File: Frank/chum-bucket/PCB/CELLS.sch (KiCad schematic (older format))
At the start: 8 parts, among them U207 CM, U208 CM, U209 CM, U210 CM, U211 CM, U212 CM, U213 CM, U214 CM

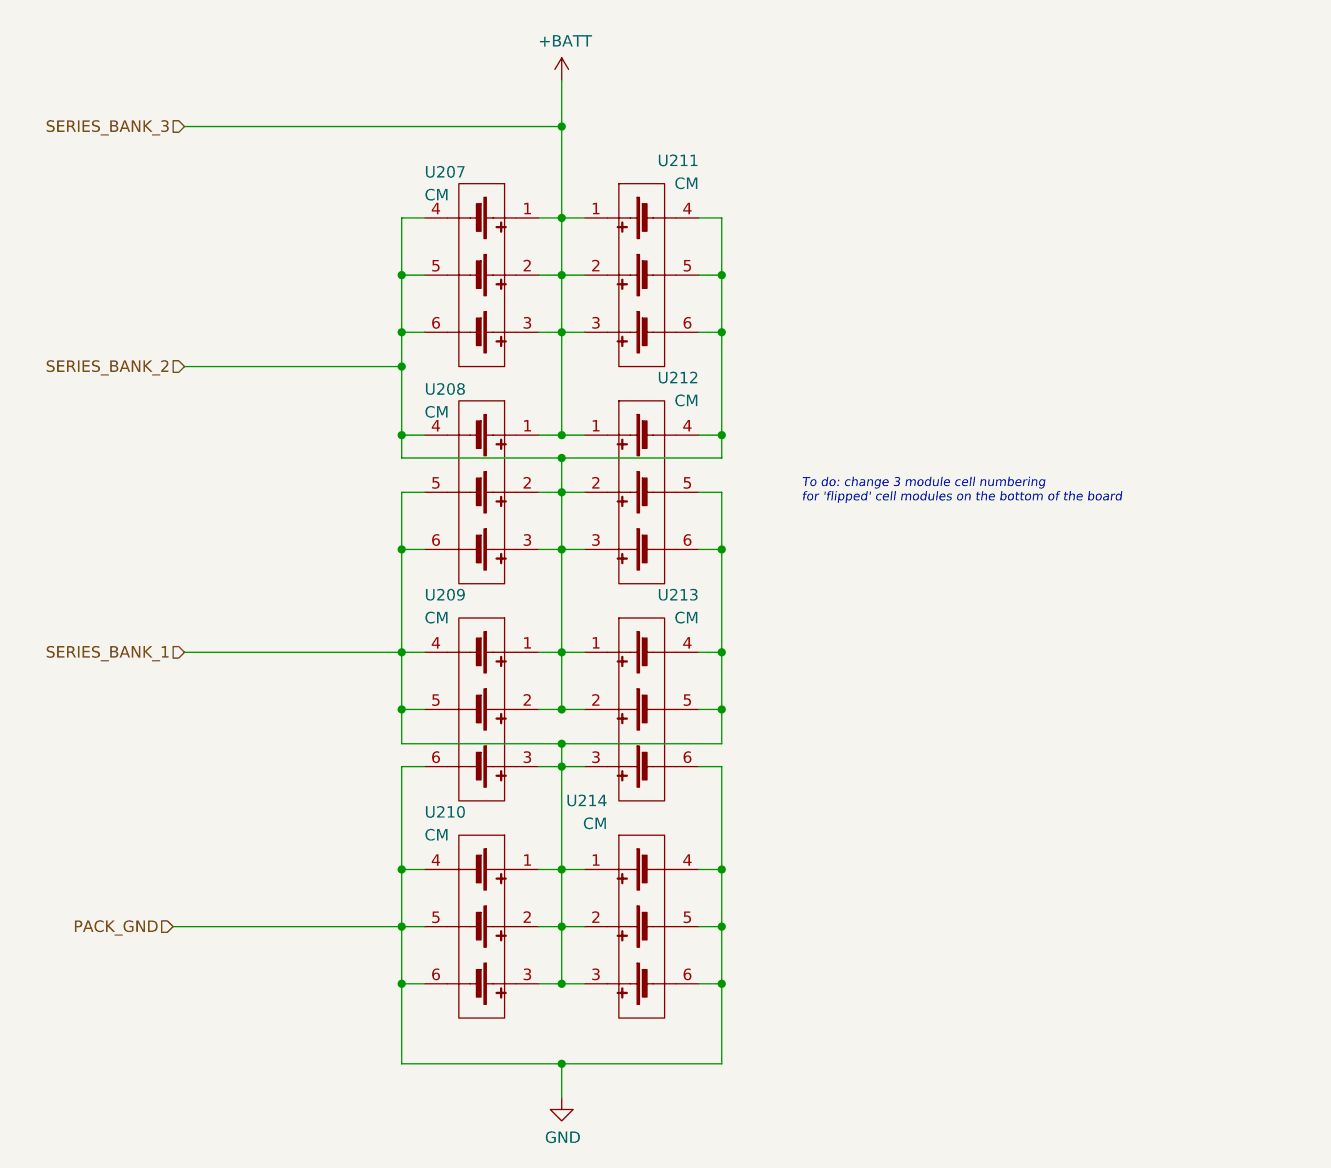
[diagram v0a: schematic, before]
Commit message: some layout
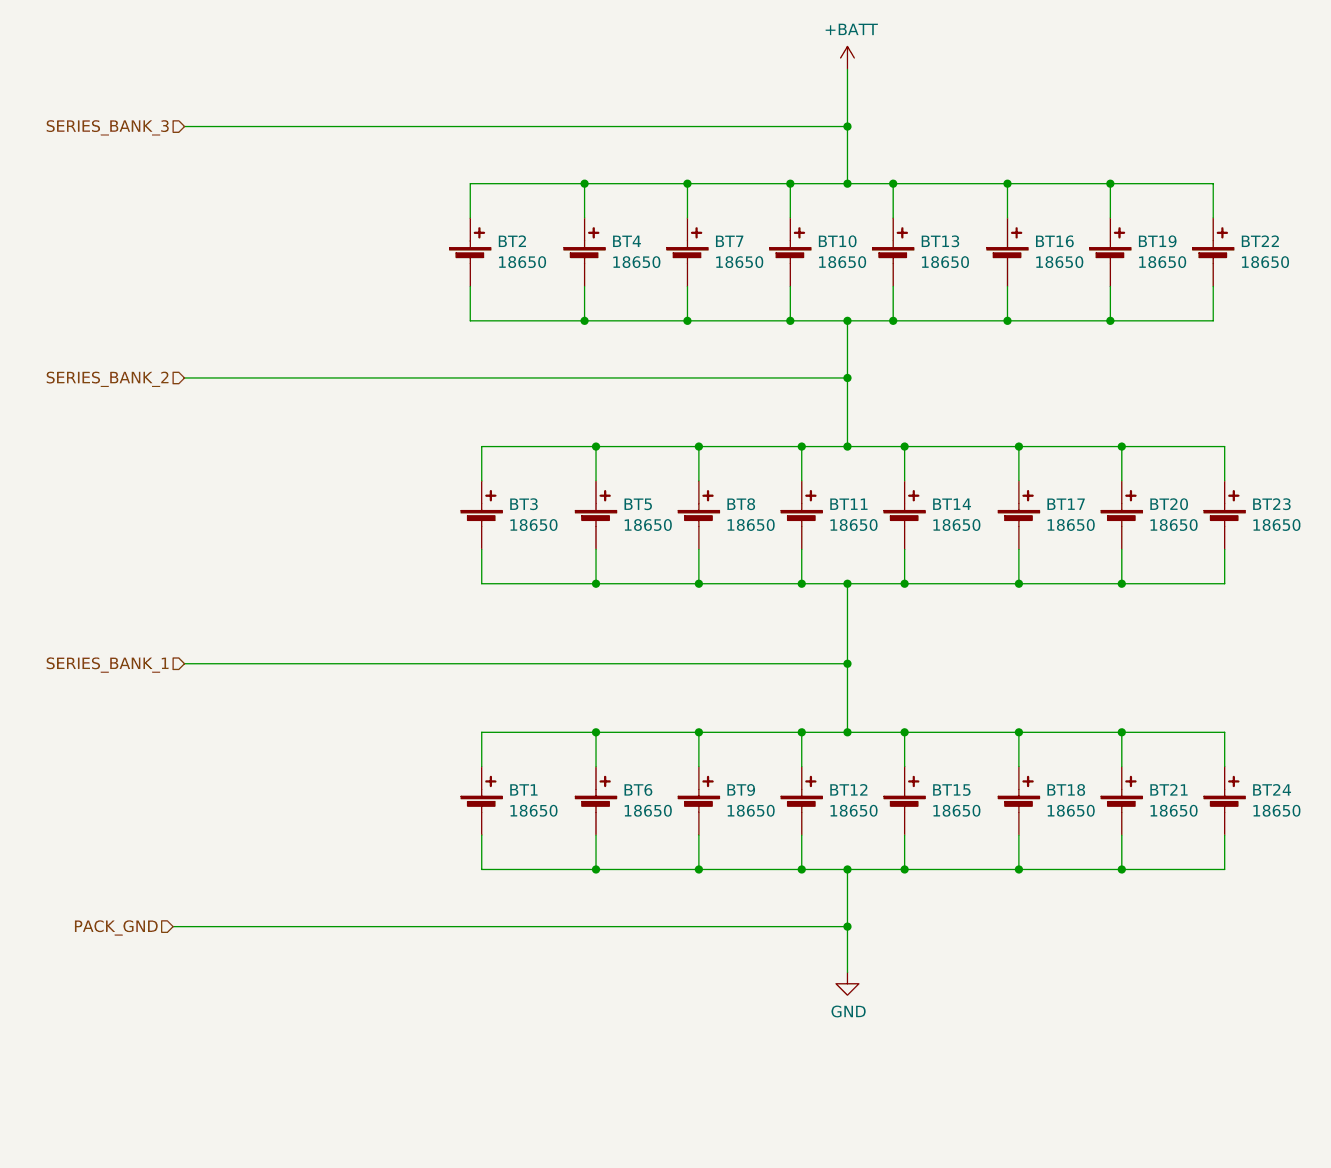
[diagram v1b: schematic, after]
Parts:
- removed U207, U208, U209, U210, U211, U212, U213, U214: CM, symbol chum-bucket:3_Cell_Module
- added BT1, BT10, BT11, BT12, BT13, BT14, BT15, BT16, BT17, BT18, BT19, BT2, BT20, BT21, BT22, BT23, BT24, BT3, BT4, BT5, BT6, BT7, BT8, BT9: 18650, CHUM_BUCKET_FOOTPRINTS:Keystone_1042p_18650_Holder, symbol Device:Battery_Cell
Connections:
- net +BATT: now also BT10.1 (+), BT13.1 (+), BT16.1 (+), BT19.1 (+), BT2.1 (+), BT22.1 (+), BT4.1 (+), BT7.1 (+)
- net GND: now also BT1.2 (-), BT12.2 (-), BT15.2 (-), BT18.2 (-), BT21.2 (-), BT24.2 (-), BT6.2 (-), BT9.2 (-)
- net SERIES_BANK_1: now also BT1.1 (+), BT11.2 (-), BT12.1 (+), BT14.2 (-), BT15.1 (+), BT17.2 (-), BT18.1 (+), BT20.2 (-), BT21.1 (+), BT23.2 (-), BT24.1 (+), BT3.2 (-), BT5.2 (-), BT6.1 (+), BT8.2 (-), BT9.1 (+)
- net SERIES_BANK_2: now also BT10.2 (-), BT11.1 (+), BT13.2 (-), BT14.1 (+), BT16.2 (-), BT17.1 (+), BT19.2 (-), BT2.2 (-), BT20.1 (+), BT22.2 (-), BT23.1 (+), BT3.1 (+), BT4.2 (-), BT5.1 (+), BT7.2 (-), BT8.1 (+)
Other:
- note removed: "To do: change 3 module cell numbering\nfor 'flipped' cell modules on the bottom of the board"
